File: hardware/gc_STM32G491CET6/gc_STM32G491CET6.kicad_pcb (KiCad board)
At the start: 2 copper layers, 108 x 88 mm, 89 parts, among them J501 Battery, J502 XL320, J503 Switch, J504 COLOR, J505 MOTOR1, J506 MOTOR2, J507 TOF, J508 FLOOR1, J509 FLOOR2, J510 GPIO1, J511 GPIO2, J512 GND, J513 GND, J514 +3.3V, J515 +3.3V, J516 +5V, J517 +5V, J7 Conn_02x07_Odd_Even, U301 STM32G070RBT6, U401 NCS199A3RSQT2G, U402 NCS199A3RSQT2G, U403 ZXBM5210-S, U404 ZXBM5210-S, U6 AZ1117CH2-5.0TRG1, U7 MIC5317-3.3YM5-TR, Y301 16MHz

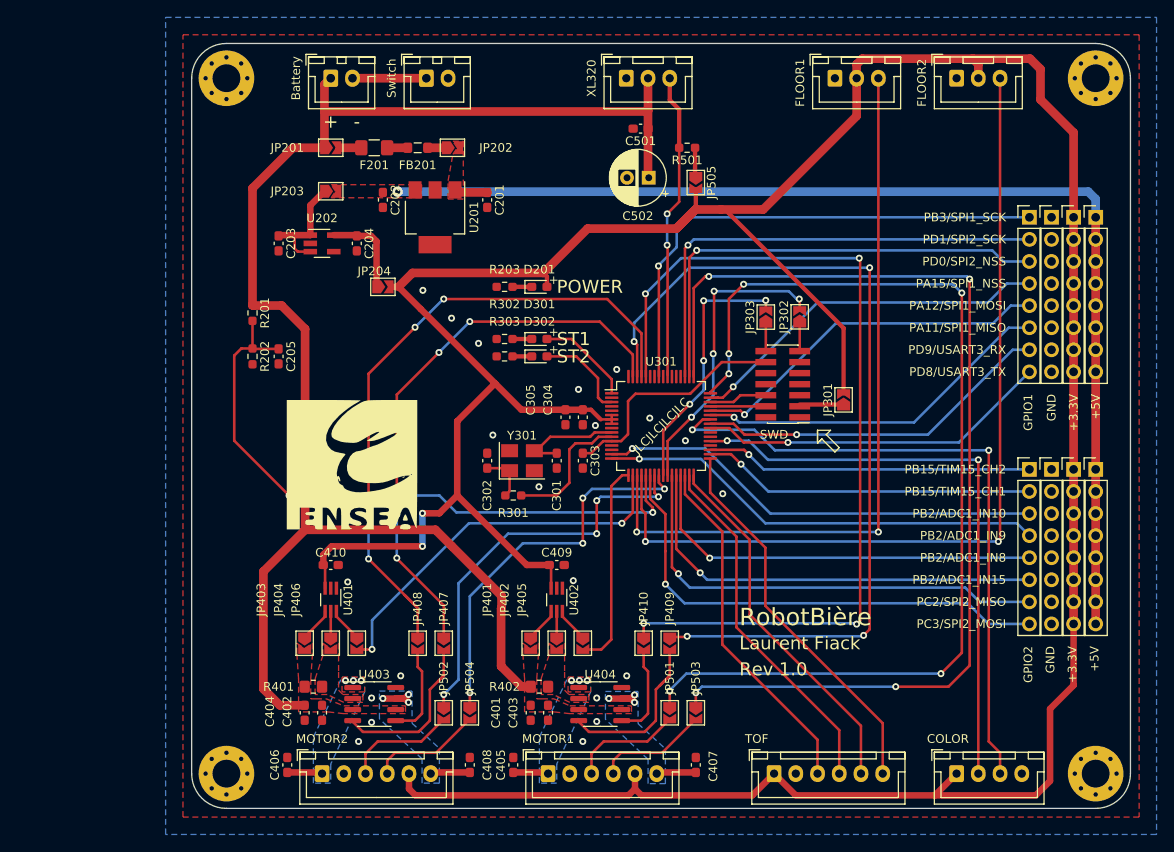
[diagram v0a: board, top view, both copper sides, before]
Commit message: Schematics + rough placement
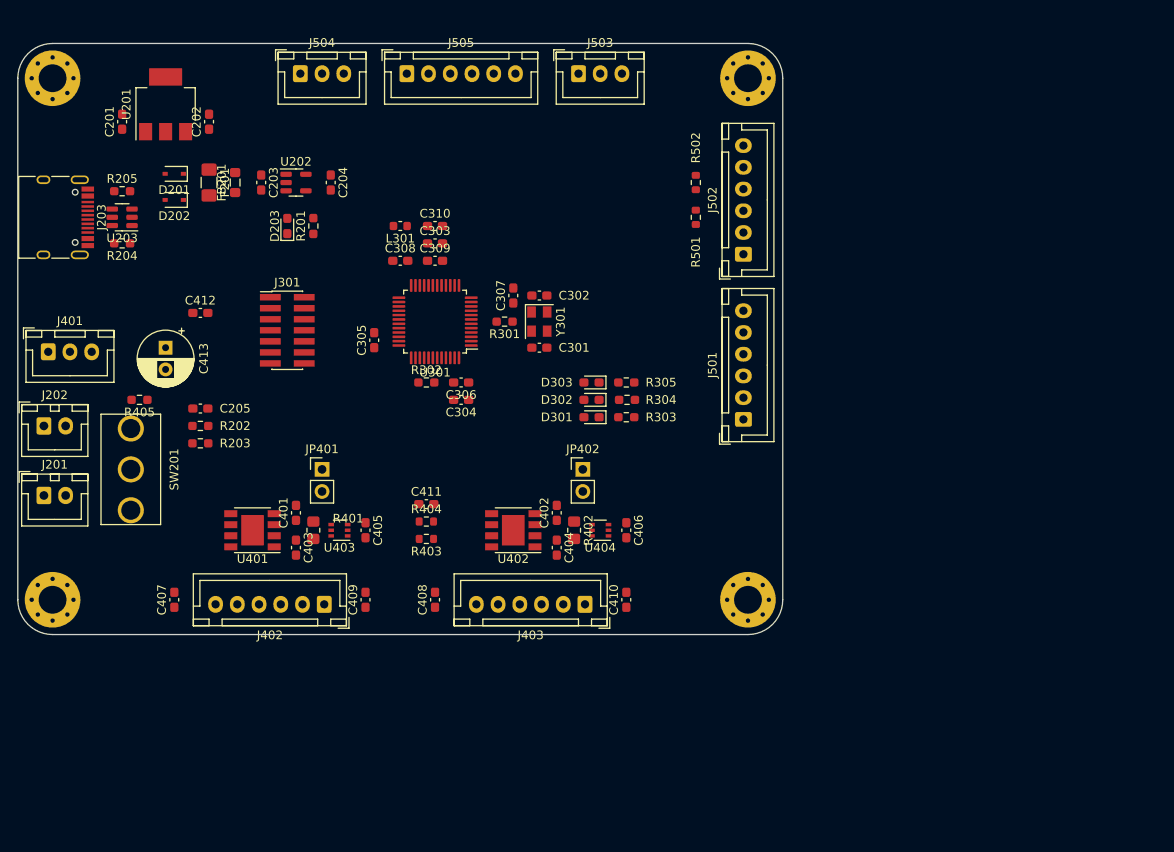
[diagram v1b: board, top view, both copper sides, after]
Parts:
- removed C403, C404, C501: 100nF, Capacitor_SMD:C_0603_1608Metric_Pad1.08x0.95mm_HandSolder
- removed C502: 100uF, Capacitor_THT:CP_Radial_D6.3mm_P2.50mm
- removed the C6 at (80.0, 44.0)
- removed the C6 at (61.0, 103.0)
- removed the C6 at (85.0, 103.0)
- removed G***: LOGO, ensea:ensea
- removed H501, H502, H503, H504: MountingHole_Pad, MountingHole:MountingHole_3.2mm_M3_Pad_Via
- removed J506: MOTOR2, Connector_JST:JST_XH_B6B-XH-A_1x06_P2.50mm_Vertical
- removed J507: TOF, Connector_JST:JST_XH_B6B-XH-A_1x06_P2.50mm_Vertical
- removed J508: FLOOR1, Connector_JST:JST_XH_B3B-XH-A_1x03_P2.50mm_Vertical
- removed J509: FLOOR2, Connector_JST:JST_XH_B3B-XH-A_1x03_P2.50mm_Vertical
- removed J510: GPIO1, Connector_PinHeader_2.54mm:PinHeader_1x08_P2.54mm_Vertical
- removed J511: GPIO2, Connector_PinHeader_2.54mm:PinHeader_1x08_P2.54mm_Vertical
- removed J512, J513: GND, Connector_PinHeader_2.54mm:PinHeader_1x08_P2.54mm_Vertical
- removed J514, J515: +3.3V, Connector_PinHeader_2.54mm:PinHeader_1x08_P2.54mm_Vertical
- removed J516, J517: +5V, Connector_PinHeader_2.54mm:PinHeader_1x08_P2.54mm_Vertical
- removed JP1, JP202, JP203, JP204, JP301, JP302, JP303, JP403, JP404, JP405, JP406, JP407, JP408, JP409, JP410, JP501, JP502, JP503, JP504, JP505: SolderJumper_2_Open, Jumper:SolderJumper-2_P1.3mm_Open_TrianglePad1.0x1.5mm
- removed U7: MIC5317-3.3YM5-TR, Package_TO_SOT_SMD:SOT-23-5_HandSoldering
- added C306: 100nF, Capacitor_SMD:C_0603_1608Metric_Pad1.08x0.95mm_HandSolder, F.Cu at (77.0, 65.0)
- added C307: 100nF, Capacitor_SMD:C_0603_1608Metric_Pad1.08x0.95mm_HandSolder, F.Cu at (83.0, 55.0)
- added C308: 100nF, Capacitor_SMD:C_0603_1608Metric_Pad1.08x0.95mm_HandSolder, F.Cu at (70.0, 51.0)
- added C309: 10nF, Capacitor_SMD:C_0603_1608Metric_Pad1.08x0.95mm_HandSolder, F.Cu at (74.0, 51.0)
- added C310: 1uF, Capacitor_SMD:C_0603_1608Metric_Pad1.08x0.95mm_HandSolder, F.Cu at (74.0, 47.0)
- added C401: 1uF, Capacitor_SMD:C_0603_1608Metric_Pad1.08x0.95mm_HandSolder, F.Cu at (58.0, 80.0)
- added C402: 1uF, Capacitor_SMD:C_0603_1608Metric_Pad1.08x0.95mm_HandSolder, F.Cu at (88.0, 80.0)
- added C411: 100nF, Capacitor_SMD:C_0603_1608Metric_Pad1.08x0.95mm_HandSolder, F.Cu at (73.0, 79.0)
- added C412: 100nF, Capacitor_SMD:C_0603_1608Metric_Pad1.08x0.95mm_HandSolder, F.Cu at (47.0, 57.0)
- added C413: 100uF, Capacitor_THT:CP_Radial_D6.3mm_P2.50mm, F.Cu at (43.0, 61.0)
- added C6: 10uF, Capacitor_SMD:C_0603_1608Metric_Pad1.08x0.95mm_HandSolder, F.Cu at (38.0, 35.0)
- added C6: 10uF, Capacitor_SMD:C_0603_1608Metric_Pad1.08x0.95mm_HandSolder, F.Cu at (58.0, 84.0)
- added C6: 10uF, Capacitor_SMD:C_0603_1608Metric_Pad1.08x0.95mm_HandSolder, F.Cu at (88.0, 84.0)
- added D202: BAT60JFILM, Diode_SMD:D_SOD-323, F.Cu at (44.0, 44.0)
- added D203: RED, LED_SMD:LED_0603_1608Metric_Pad1.05x0.95mm_HandSolder, F.Cu at (57.0, 47.0)
- added D303: BLUE, LED_SMD:LED_0603_1608Metric_Pad1.05x0.95mm_HandSolder, F.Cu at (92.0, 65.0)
- added H101: MountingHole_3.2mm_M3_Pad_Via, MountingHole:MountingHole_3.2mm_M3_Pad_Via, F.Cu at (30.0, 90.0)
- added H102: MountingHole_3.2mm_M3_Pad_Via, MountingHole:MountingHole_3.2mm_M3_Pad_Via, F.Cu at (30.0, 30.0)
- added H103: MountingHole_3.2mm_M3_Pad_Via, MountingHole:MountingHole_3.2mm_M3_Pad_Via, F.Cu at (110.0, 30.0)
- added H104: MountingHole_3.2mm_M3_Pad_Via, MountingHole:MountingHole_3.2mm_M3_Pad_Via, F.Cu at (110.0, 90.0)
- added J201: Battery, Connector_JST:JST_XH_B2B-XH-A_1x02_P2.50mm_Vertical, F.Cu at (29.0, 78.0)
- added J202: Recharge, Connector_JST:JST_XH_B2B-XH-A_1x02_P2.50mm_Vertical, F.Cu at (29.0, 70.0)
- added J203: USB_C_Receptacle_USB2.0, Connector_USB:USB_C_Receptacle_HRO_TYPE-C-31-M-12, F.Cu at (30.0, 46.0)
- added J401: XL320, Connector_JST:JST_XH_B3B-XH-A_1x03_P2.50mm_Vertical, F.Cu at (29.5, 61.5)
- added J402: MOTOR1, Connector_JST:JST_XH_B6B-XH-A_1x06_P2.50mm_Vertical, F.Cu at (61.2, 90.5)
- added J403: MOTOR2, Connector_JST:JST_XH_B6B-XH-A_1x06_P2.50mm_Vertical, F.Cu at (91.2, 90.5)
- added L301: 39nH, Inductor_SMD:L_0603_1608Metric, F.Cu at (70.0, 47.0)
- added R204: 5.1k, Resistor_SMD:R_0603_1608Metric_Pad0.98x0.95mm_HandSolder, F.Cu at (38.0, 49.0)
- added R205: 5.1k, Resistor_SMD:R_0603_1608Metric_Pad0.98x0.95mm_HandSolder, F.Cu at (38.0, 43.0)
- added R304: 1k, Resistor_SMD:R_0603_1608Metric_Pad0.98x0.95mm_HandSolder, F.Cu at (96.1, 67.0)
- added R305: 1k, Resistor_SMD:R_0603_1608Metric_Pad0.98x0.95mm_HandSolder, F.Cu at (96.0, 65.0)
- added R403: 100k, Resistor_SMD:R_0603_1608Metric, F.Cu at (73.0, 83.0)
- added R404: 100k, Resistor_SMD:R_0603_1608Metric, F.Cu at (73.0, 81.0)
- added R405: 10k, Resistor_SMD:R_0603_1608Metric_Pad0.98x0.95mm_HandSolder, F.Cu at (40.0, 67.0)
- added R502: 2.2k, Resistor_SMD:R_0603_1608Metric, F.Cu at (104.0, 42.0)
- added SW201: ON/OFF, WITNS:RS_Switch_448-0747, F.Cu at (39.0, 75.0)
- added U202: BU33SD5WG-TR, Package_TO_SOT_SMD:SOT-23-5, F.Cu at (58.0, 42.0)
- added U203: USBLC6-2SC6, Package_TO_SOT_SMD:SOT-23-6, F.Cu at (38.0, 46.0)
- C304: value 100nF -> 4.7uF
- C305: value 4.7uF -> 100nF
- D201: value RED -> BAT60JFILM; footprint LED_SMD:LED_0603_1608Metric_Pad1.05x0.95mm_HandSolder -> Diode_SMD:D_SOD-323
- D301: value GREEN -> RED
- D302: value RED -> GREEN
- J501: value Battery -> TOF1; footprint Connector_JST:JST_XH_B2B-XH-A_1x02_P2.50mm_Vertical -> Connector_JST:JST_XH_B6B-XH-A_1x06_P2.50mm_Vertical
- J502: value XL320 -> TOF2; footprint Connector_JST:JST_XH_B3B-XH-A_1x03_P2.50mm_Vertical -> Connector_JST:JST_XH_B6B-XH-A_1x06_P2.50mm_Vertical
- J503: value Switch -> FLOOR1; footprint Connector_JST:JST_XH_B2B-XH-A_1x02_P2.50mm_Vertical -> Connector_JST:JST_XH_B3B-XH-A_1x03_P2.50mm_Vertical
- J504: value COLOR -> FLOOR2; footprint Connector_JST:JST_XH_B4B-XH-A_1x04_P2.50mm_Vertical -> Connector_JST:JST_XH_B3B-XH-A_1x03_P2.50mm_Vertical
- J505: value MOTOR1 -> TCS3200
- JP401, JP402: value SolderJumper_2_Open -> Jumper_2_Open; footprint Jumper:SolderJumper-2_P1.3mm_Open_TrianglePad1.0x1.5mm -> Connector_PinHeader_2.54mm:PinHeader_1x02_P2.54mm_Vertical
- R201: value 220k -> 1k
- R202: value 100k -> 220k
- R203, R302: value 1k -> 100k
- R501: value 10k -> 2.2k; footprint Resistor_SMD:R_0603_1608Metric_Pad0.98x0.95mm_HandSolder -> Resistor_SMD:R_0603_1608Metric
- U301: value STM32G070RBT6 -> STM32G491CET6; footprint Package_QFP:LQFP-64_10x10mm_P0.5mm -> Package_QFP:LQFP-48_7x7mm_P0.5mm
- U401, U402: value NCS199A3RSQT2G -> ZXBM5210-SP; footprint Package_TO_SOT_SMD:SOT-363_SC-70-6_Handsoldering -> Package_SO:Diodes_SO-8EP
- U403, U404: value ZXBM5210-S -> NCS199A3RSQT2G; footprint Package_SO:SOIC-8_3.9x4.9mm_P1.27mm -> Package_TO_SOT_SMD:SOT-363_SC-70-6
- Y301: footprint Crystal:Crystal_SMD_EuroQuartz_MT-4Pin_3.2x2.5mm_HandSoldering -> Crystal:Crystal_SMD_EuroQuartz_MT-4Pin_3.2x2.5mm
- moved J504 110.4 mm to (58.5, 29.5)
- moved J505 82.1 mm to (70.8, 29.5)
- moved C407 62.9 mm to (44.0, 90.0)
- moved J501 61.6 mm to (109.5, 69.2), turned to 90 degrees
- moved J7 57.3 mm to (57.0, 59.0), turned to 0 degrees
- moved C406 47.4 mm to (96.0, 82.0), turned to -90 degrees
- moved D201 44.0 mm to (44.0, 41.0), turned to 180 degrees
- moved R203 39.4 mm to (47.0, 72.0)
- moved C410 34.2 mm to (96.0, 90.0), turned to 90 degrees
- moved U6 33.6 mm to (43.0, 33.0), turned to 90 degrees
- moved C405 31.9 mm to (66.0, 82.0), turned to -90 degrees
- moved JP401 31.2 mm to (61.0, 75.0), turned to 0 degrees
- moved C303 30.2 mm to (74.0, 49.0), turned to 0 degrees
- moved U301 28.6 mm to (74.0, 58.0), turned to 180 degrees
- moved J502 24.3 mm to (109.5, 50.2), turned to 90 degrees
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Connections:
- net I2C_COLOR_SDA renamed /STM32/FLOOR_2
- net Net-(C302-Pad2) renamed /STM32/XTAL1
- net Net-(F201-Pad2) renamed /Power Supply/FUSE
- net STATUS_LED_R renamed /STM32/STATUS_LED_G
- C203 pad 1: /Power Supply/3.3_VIN -> /Power Supply/BU33_IN
- C204 pad 1: /Power Supply/3.3_VOUT -> +3.3V
- C205 pad 1: BAT_SENSE -> /Power Supply/BAT_SENSE
- C303 pad 1: NRST -> +3.3VA
- C304 pad 1: +3V3 -> +3.3V
- C305 pad 1: +3V3 -> +3.3V
- C405 pad 1: MOTOR1_OUT1 -> +3.3V
- C406 pad 1: MOTOR2_OUT1 -> +3.3V
- C407 pad 1: MOTOR1_OUT2 -> /Actuators/M1_OUT2
- C408 pad 1: MOTOR2_OUT2 -> /Actuators/M2_OUT2
- C409 pad 1: +3V3 -> /Actuators/M1_OUT1
- C410 pad 1: +3V3 -> /Actuators/M2_OUT1
- D201 pad 1: Net-(D201-Pad1) -> /Power Supply/KATHODES
- D201 pad 2: +3V3 -> +5V
- D301 pad 2: STATUS_LED_G -> /STM32/STATUS_LED_R
- F201 pad 1: Net-(F201-Pad1) -> /Power Supply/KATHODES
- FB1 pad 2: Net-(FB201-Pad2) -> /Power Supply/BU33_IN
- J501 pad 1: +BATT -> +3.3V
- J501 pad 2: /Connectors/BAT_Middle -> GND
- J502 pad 1: GND -> +3.3V
- J502 pad 2: +BATT -> GND
- J502 pad 3: XL320 -> /STM32/TOF_I2C_SDA
- J503 pad 1: /Connectors/BAT_Middle -> GND
- J503 pad 2: GND -> +3.3V
- J504 pad 1: +3V3 -> GND
- J504 pad 2: I2C_COLOR_SCL -> +3.3V
- J505 pad 1: MOTOR1_OUT1 -> +3.3V
- J505 pad 2: GND -> /STM32/TCS3200_TIM
- J505 pad 3: Net-(J505-Pad3) -> /STM32/TCS3200_LED
- J505 pad 4: Net-(J505-Pad4) -> /STM32/TCS3200_S3
- J505 pad 5: +3V3 -> /STM32/TCS3200_S2
- J505 pad 6: MOTOR1_OUT2 -> GND
- J7 pad 12: NRST -> /STM32/NRST
- J7 pad 13: Net-(J301-Pad13) -> /STM32/STLINK_RX
- J7 pad 14: Net-(J301-Pad14) -> /STM32/STLINK_TX
- J7 pad 3: Net-(J301-Pad3) -> +3.3V
- J7 pad 4: SWDIO -> /STM32/SWDIO
- J7 pad 6: SWCLK -> /STM32/SWCLK
- J7 pad 8: unconnected-(J301-Pad8) -> /STM32/SWO
- JP401 pad 1: Net-(JP401-Pad1) -> +BATT
- JP401 pad 2: +BATT -> /Actuators/M1_VDD
- JP402 pad 1: Net-(JP402-Pad1) -> +BATT
- JP402 pad 2: VM1 -> /Actuators/M2_VDD
- R201 pad 1: +BATT -> Net-(D203-Pad1)
- R201 pad 2: BAT_SENSE -> GND
- R202 pad 1: BAT_SENSE -> +BATT
- R202 pad 2: GND -> /Power Supply/BAT_SENSE
- R203 pad 1: Net-(D201-Pad1) -> /Power Supply/BAT_SENSE
- R302 pad 1: Net-(D301-Pad1) -> GND
- R302 pad 2: GND -> /STM32/BOOT0
- R303 pad 1: Net-(D302-Pad1) -> Net-(D301-Pad1)
- R401 pad 1: +BATT -> /Actuators/M1_VDD
- R401 pad 2: VM2 -> /Actuators/M1_VM
- R402 pad 1: +BATT -> /Actuators/M2_VDD
- R402 pad 2: VM1 -> /Actuators/M2_VM
- R501 pad 1: Net-(JP505-Pad1) -> +3.3V
- R501 pad 2: XL320 -> /STM32/TOF_I2C_SDA
- U301 pad 1: STATUS_LED_G -> +3.3V
- U301 pad 10: /STM32/OSC_IN -> /STM32/STLINK_TX
- U301 pad 11: /STM32/OSC_OUT -> /STM32/STLINK_RX
- U301 pad 12: NRST -> /Actuators/M1_ENC_A
- U301 pad 13: unconnected-(U301-Pad13) -> /Actuators/M1_TIM_FWD
- U301 pad 14: unconnected-(U301-Pad14) -> /Actuators/M1_ENC_B
- U301 pad 15: PC2/SPI2_MISO -> /STM32/TOF1_XSHUT
- U301 pad 16: PC3/SPI2_MOSI -> /STM32/TOF1_GPIO1
- U301 pad 17: DCMOTOR1_ISENSE -> /STM32/TOF2_XSHUT
- U301 pad 18: DCMOTOR2_ISENSE -> /STM32/TOF2_GPIO1
- U301 pad 19: FLOOR_SENSOR1 -> GND
- U301 pad 2: unconnected-(U301-Pad2) -> /STM32/STATUS_LED_R
- U301 pad 20: FLOOR_SENSOR2 -> +3.3VA
- U301 pad 21: BAT_SENSE -> +3.3VA
- U301 pad 22: PA5/ADC1_IN15 -> /Actuators/M2_TIM_FWD
- U301 pad 23: ENCODER2_A -> GND
- U301 pad 24: ENCODER2_B -> +3.3V
- U301 pad 25: VCP_TX -> /STM32/TCS3200_LED
- U301 pad 26: VCP_RX -> /Actuators/M2_ADC_ISENSE
- U301 pad 27: PB0/ADC1_IN8 -> /STM32/TCS3200_S3
- U301 pad 28: PB1/ADC1_IN9 -> /Power Supply/BAT_SENSE
- U301 pad 29: PB2/ADC1_IN10 -> /STM32/TCS3200_S2
- U301 pad 30: I2C_TOF_SDA -> /STM32/TOF_I2C_SDA
- U301 pad 31: I2C_TOF_SCL -> /STM32/TOF_I2C_SCL
- U301 pad 32: TOF_XSHUT -> /Actuators/M2_TIM_REV
- U301 pad 33: TOF_GPIO1 -> /Power Supply/USB_DM
- U301 pad 34: PB14/TIM15_CH1 -> /Power Supply/USB_DP
- U301 pad 35: PB15/TIM15_CH2 -> GND
- U301 pad 36: unconnected-(U301-Pad36) -> +3.3V
- U301 pad 37: I2C_COLOR_SCL -> /STM32/SWDIO
- U301 pad 38: unconnected-(U301-Pad38) -> /STM32/SWCLK
- U301 pad 39: unconnected-(U301-Pad39) -> /STM32/FLOOR_1
- U301 pad 4: unconnected-(U301-Pad4) -> /STM32/STATUS_LED_B
- U301 pad 40: PD8/USART3_TX -> /STM32/SWO
- U301 pad 41: PD9/USART3_RX -> /STM32/TCS3200_TIM
- U301 pad 43: PA11/SPI1_MISO -> /Actuators/M2_ENC_A
- U301 pad 44: PA12/SPI1_MOSI -> /Actuators/M2_ENC_B
- U301 pad 45: SWDIO -> /STM32/BOOT0
- U301 pad 46: SWCLK -> /Actuators/XL320_UART
- U301 pad 47: PA15/SPI1_NSS -> GND
- U301 pad 48: ENCODER1_A -> +3.3V
- U301 pad 5: unconnected-(U301-Pad5) -> /STM32/OSC_IN
- U301 pad 6: +3V3 -> /STM32/OSC_OUT
- U301 pad 7: +3V3 -> /STM32/NRST
- U301 pad 8: +3V3 -> /Actuators/M1_ADC_ISENSE
- U301 pad 9: GND -> /Actuators/M1_TIM_REV
- U401 pad 1: GND -> /Actuators/M1_OUT1
- U401 pad 2: GND -> /Actuators/M1_VM
- U401 pad 3: +3V3 -> /Actuators/M1_VDD
- U401 pad 4: Net-(JP403-Pad1) -> /Actuators/M1_TIM_FWD
- U401 pad 5: Net-(JP404-Pad1) -> /Actuators/M1_TIM_REV
- U401 pad 6: Net-(JP406-Pad1) -> /Actuators/M1_VDD
- U402 pad 1: GND -> /Actuators/M2_OUT1
- U402 pad 2: GND -> /Actuators/M2_VM
- U402 pad 3: +3V3 -> /Actuators/M2_VDD
- U402 pad 4: Net-(JP401-Pad1) -> /Actuators/M2_TIM_FWD
- U402 pad 5: Net-(JP402-Pad1) -> /Actuators/M2_TIM_REV
- U402 pad 6: Net-(JP405-Pad1) -> /Actuators/M2_VDD
- U403 pad 1: MOTOR2_OUT1 -> /Actuators/NCS_REF
- U403 pad 2: VM2 -> GND
- U403 pad 3: +BATT -> +3.3V
- U403 pad 4: Net-(JP407-Pad2) -> /Actuators/M1_VDD
- U403 pad 5: Net-(JP408-Pad2) -> /Actuators/M1_VM
- U403 pad 6: +BATT -> /Actuators/M1_ADC_ISENSE
- U404 pad 1: MOTOR1_OUT1 -> /Actuators/NCS_REF
- U404 pad 2: VM1 -> GND
- U404 pad 3: +BATT -> +3.3V
- U404 pad 4: Net-(JP409-Pad2) -> /Actuators/M2_VDD
- U404 pad 5: Net-(JP410-Pad2) -> /Actuators/M2_VM
- U404 pad 6: +BATT -> /Actuators/M2_ADC_ISENSE
- U6 pad 1: VCC -> +BATT
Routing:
- net +3V3: track 383.3 -> 0.00 mm, vias 2 -> 0
- net +BATT: track 175.0 -> 0.00 mm
- net +5V: track 129.5 -> 0.00 mm, vias 1 -> 0
- net ENCODER1_B: track 121.4 -> 0.00 mm, vias 4 -> 0
- net ENCODER1_A: track 118.3 -> 0.00 mm, vias 6 -> 0
- net MOTOR1_PWM_N: track 104.3 -> 0.00 mm, vias 4 -> 0
- net FLOOR_SENSOR2: track 101.8 -> 0.00 mm, vias 2 -> 0
- net MOTOR1_PWM: track 101.0 -> 0.00 mm, vias 4 -> 0
- net FLOOR_SENSOR1: track 86.5 -> 0.00 mm, vias 2 -> 0
- net MOTOR2_PWM_N: track 76.3 -> 0.00 mm, vias 4 -> 0
- net /STM32/FLOOR_2: track 75.3 -> 0.00 mm, vias 2 -> 0
- net BAT_SENSE: track 74.6 -> 0.00 mm, vias 2 -> 0
- net I2C_COLOR_SCL: track 67.9 -> 0.00 mm, vias 2 -> 0
- net MOTOR2_PWM: track 64.8 -> 0.00 mm, vias 4 -> 0
- net PB3/SPI1_SCK: track 58.8 -> 0.00 mm, vias 1 -> 0
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- removed copper zone on F.Cu, net +5V
- removed copper zone on F.Cu, net +BATT
- removed copper zone on B.Cu, net GND
- removed copper zone on F.Cu, net GND
- removed copper zone on B.Cu, net MOTOR1_OUT1
- removed copper zone on F.Cu, net MOTOR1_OUT1
- removed copper zone on B.Cu, net MOTOR1_OUT2
- removed copper zone on B.Cu, net MOTOR2_OUT1
- removed copper zone on F.Cu, net MOTOR2_OUT1
- removed copper zone on B.Cu, net MOTOR2_OUT2
- removed copper zone on F.Cu, net VCC
- removed copper zone on F.Cu, net VM1
- removed copper zone on F.Cu, net VM2
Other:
- board size 108 x 88 mm -> 88 x 68 mm
- board text removed: "+"
- board text removed: "-"
- board text removed: "JLCJLCJLCJLC"
- board text removed: "Laurent Fiack"
- board text removed: "PA11/SPI1_MISO"
- board text removed: "PA12/SPI1_MOSI"
- board text removed: "PA15/SPI1_NSS"
- board text removed: "PB15/TIM15_CH1"
- board text removed: "PB15/TIM15_CH2"
- board text removed: "PB2/ADC1_IN10"
- board text removed: "PB2/ADC1_IN15"
- board text removed: "PB2/ADC1_IN8"
- board text removed: "PB2/ADC1_IN9"
- board text removed: "PB3/SPI1_SCK"
- board text removed: "PC2/SPI2_MISO"
- board text removed: "PC3/SPI2_MOSI"
- board text removed: "PD0/SPI2_NSS"
- board text removed: "PD1/SPI2_SCK"
- board text removed: "PD8/USART3_TX"
- board text removed: "PD9/USART3_RX"
- board text removed: "POWER"
- board text removed: "Rev 1.0"
- board text removed: "RobotBière"
- board text removed: "ST1"
- board text removed: "ST2"
